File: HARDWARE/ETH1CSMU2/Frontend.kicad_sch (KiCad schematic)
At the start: 41 parts, among them U601 DG419DY, U602 DG419DY, U603 SN74LVC1T45DRLR, U604 SN74LVC1T45DRLR, U605 LT1970ACFE, U606 SN74LVC1T45DRLR, U607 INA823DT

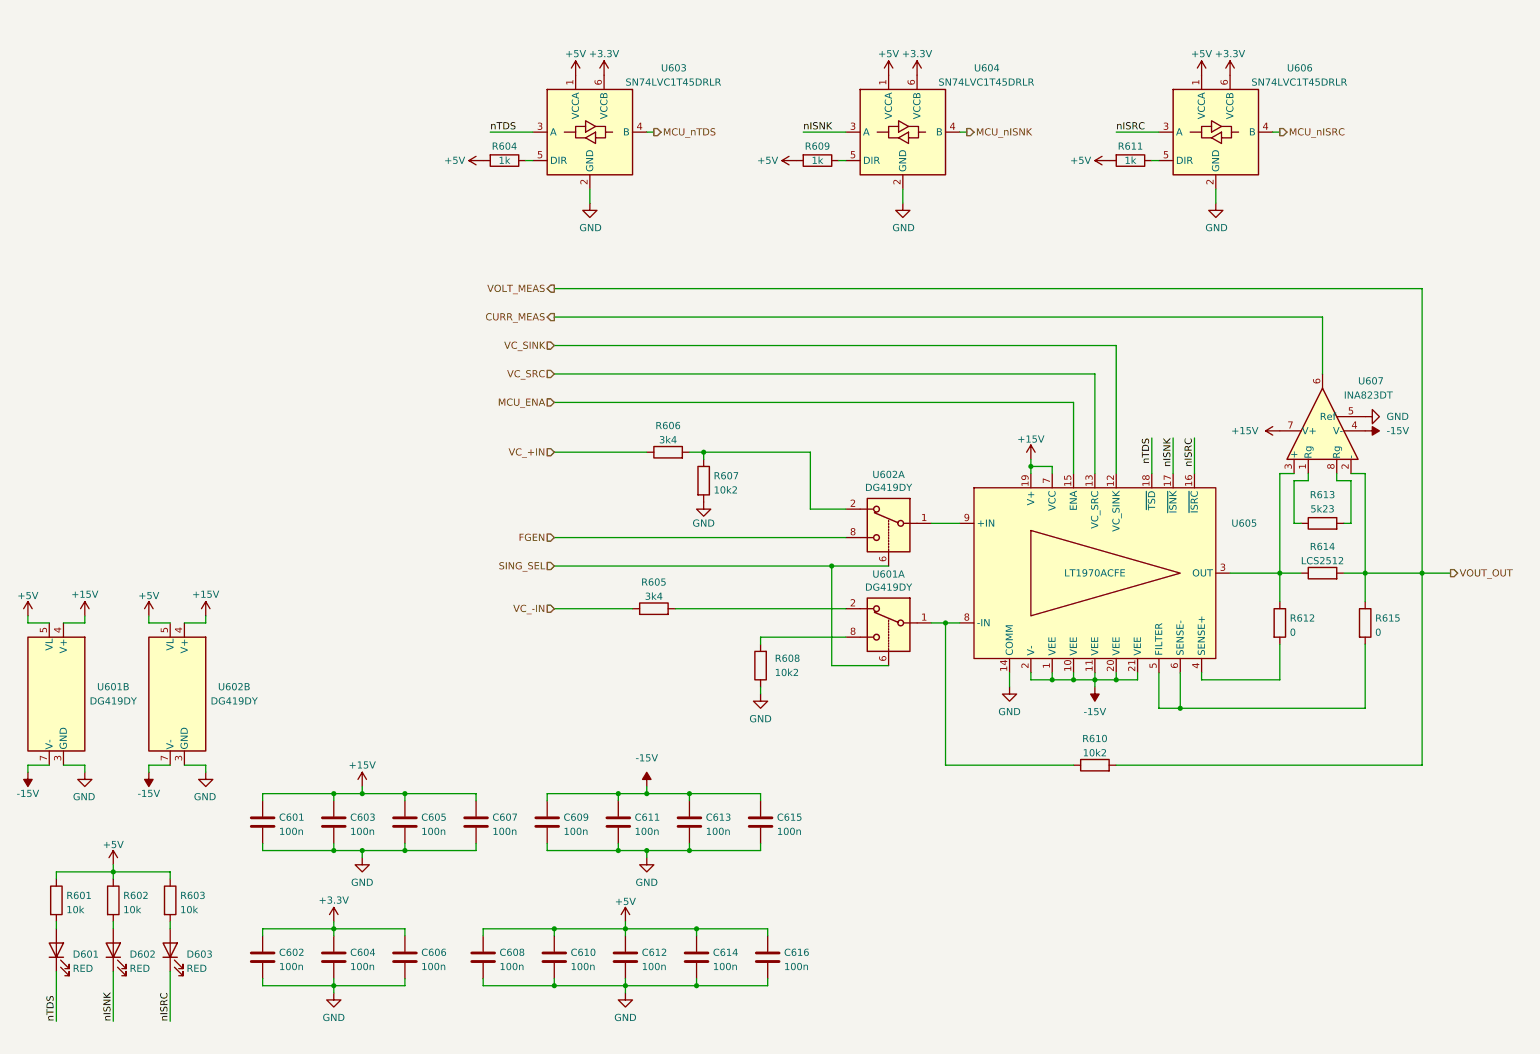
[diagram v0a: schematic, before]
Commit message: Hardware design
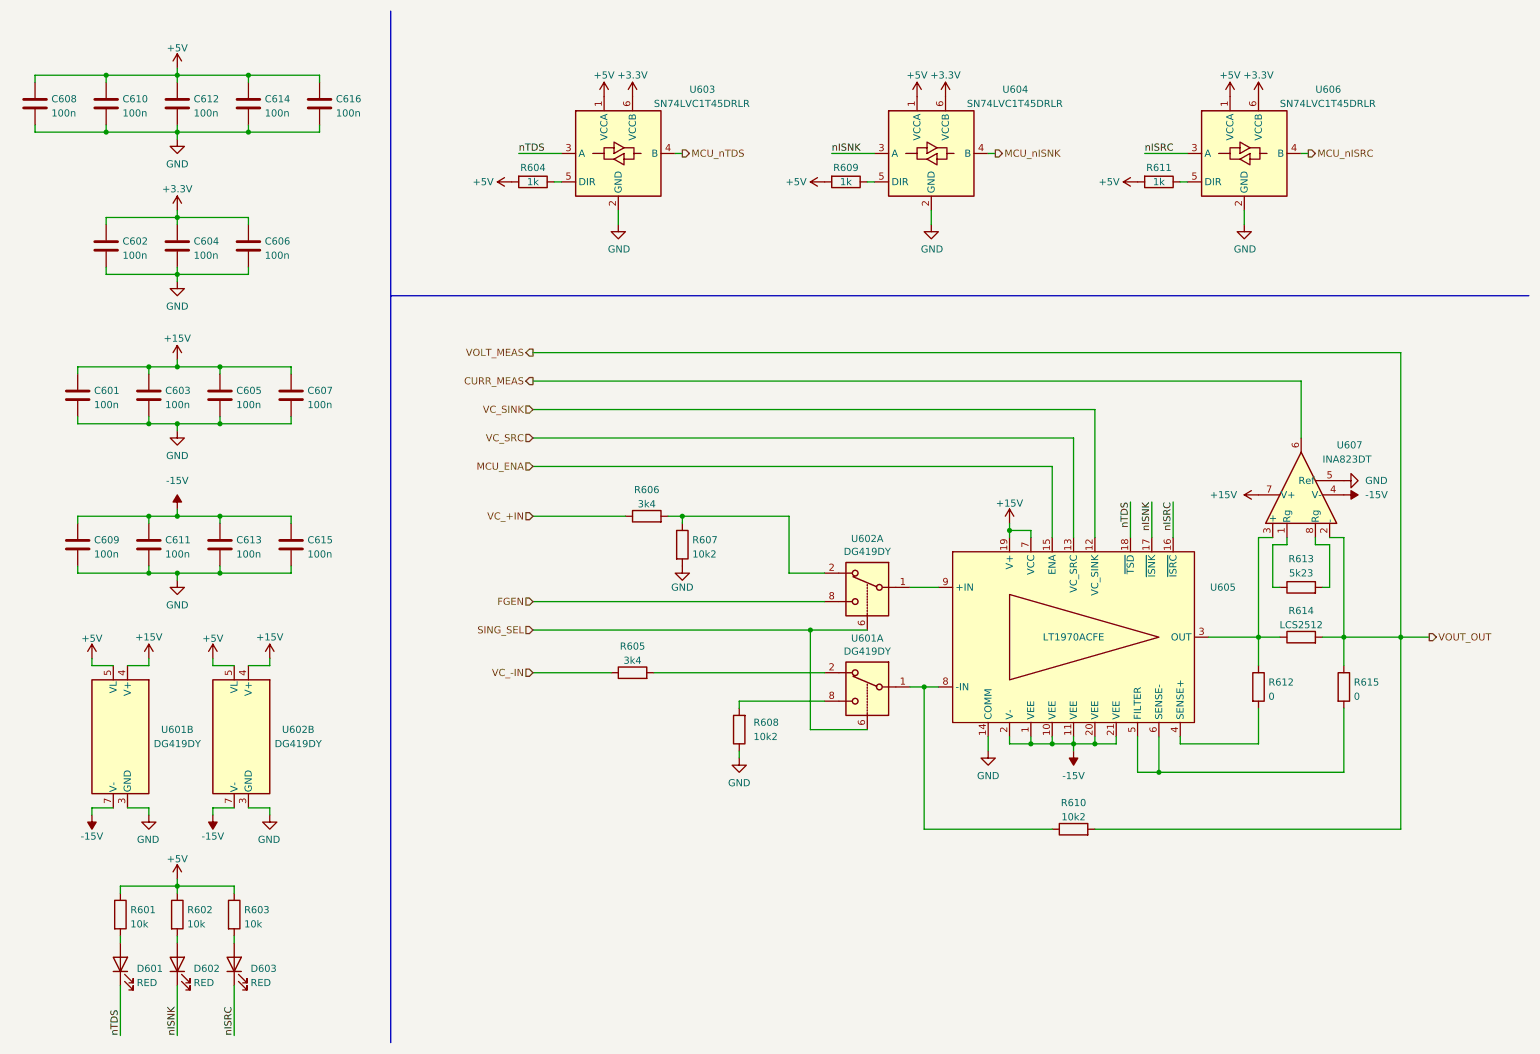
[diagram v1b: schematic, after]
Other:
- moved on the sheet: C601, C602, C603, C604, C605, C606, C607, C608, C609, C610, C611, C612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
